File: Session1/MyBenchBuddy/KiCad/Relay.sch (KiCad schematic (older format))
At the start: 0 parts

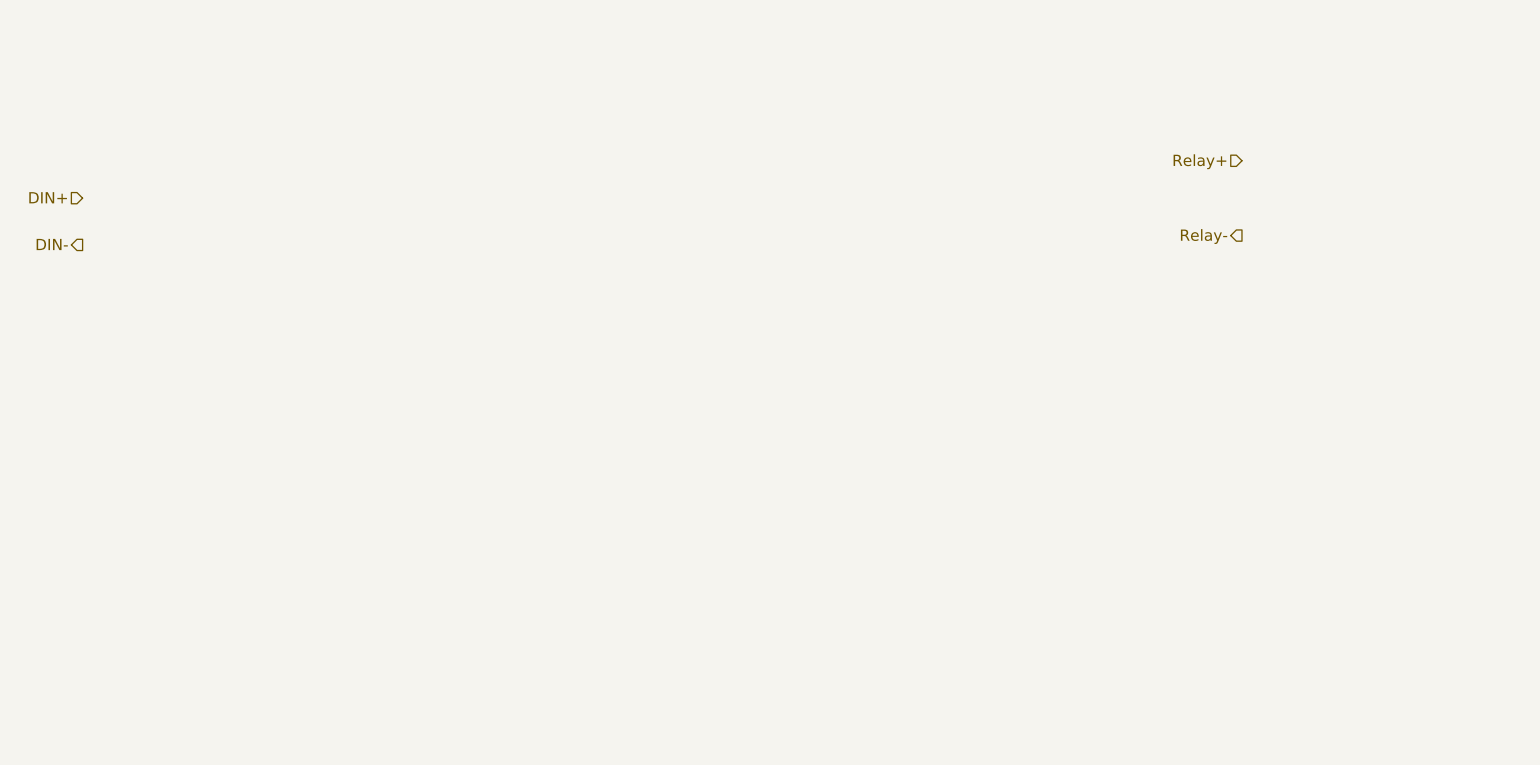
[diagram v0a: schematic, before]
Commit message: Module3Unit5
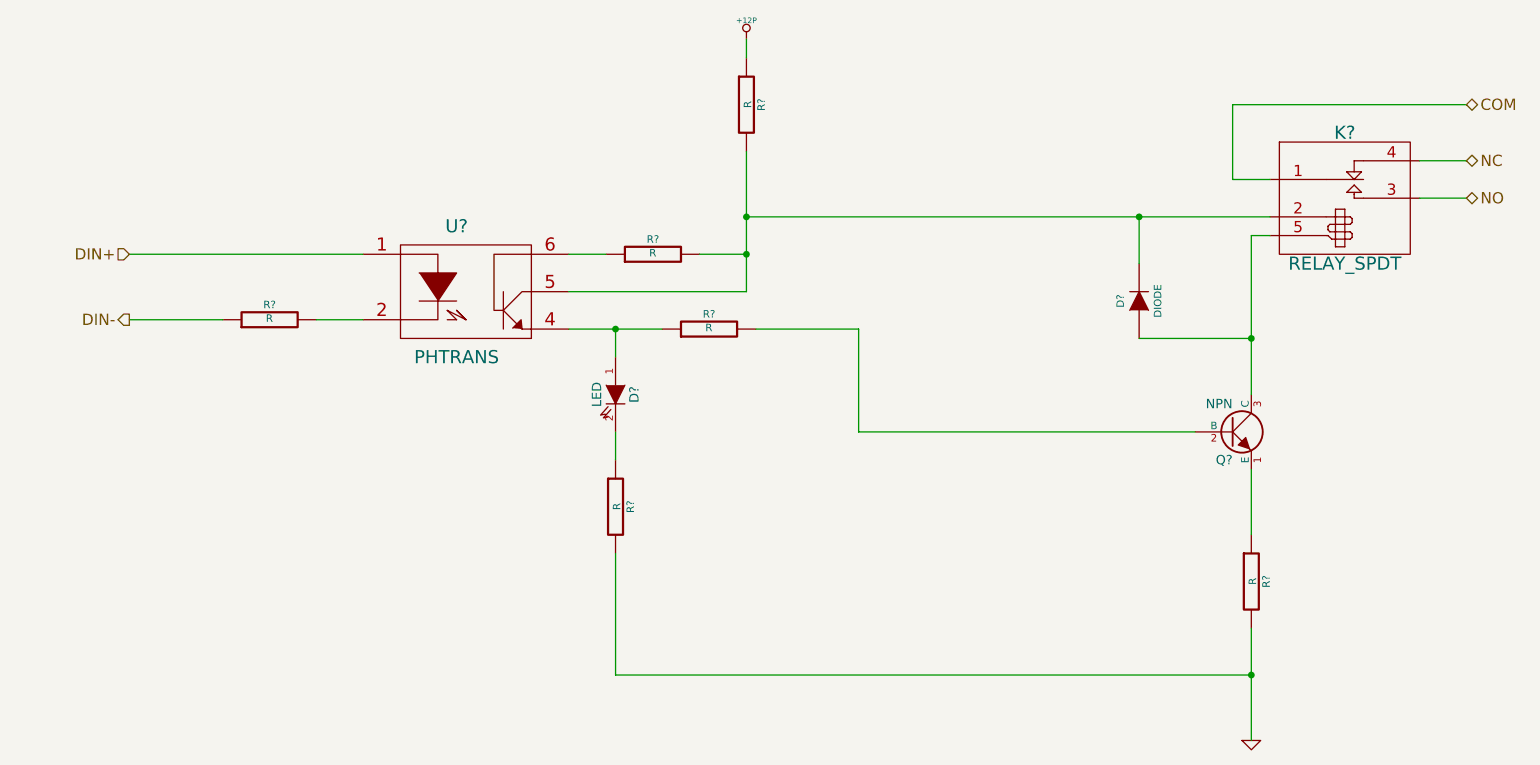
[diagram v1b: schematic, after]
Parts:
- added D?: LED, symbol LED
- added D?: DIODE, symbol DIODE
- added K?: RELAY_SPDT, symbol RELAY_SPDT
- added Q?: NPN, symbol NPN
- added R? (x6): R, symbol R
- added U?: PHTRANS, symbol PHTRANS
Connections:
- net DIN+: now also U?.1
- net DIN-: now also R?.1
- new net: R?.2, U?.2
- new net: D?.1 (A), R?.1, U?.4
- new net: D?.2 (K), K?.2 (COIL+), R?.2, R?.2, U?.5
- new net: R?.1, U?.6
- new net: Q?.2 (B), R?.2
- new net: Q?.1 (E), R?.1
- new net: D?.1 (A), K?.5 (COIL-), Q?.3 (C)
- new net: D?.2 (K), R?.1
- new net +12P: R?.1
- new net COM: K?.1 (COM)
- new net GND: R?.2, R?.2
- new net NC: K?.4 (NC)
- new net NO: K?.3 (NO)
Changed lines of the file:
@@
 LIBS:contrib
 LIBS:valves
+LIBS:bth-switch
 LIBS:MyBenchBuddy-cache
 EELAYER 24 0
@@
 $Descr A4 11693 8268
 encoding utf-8
-Sheet 4 8
+Sheet 8 8
 Title ""
 Date ""
@@
 Comment4 ""
 $EndDescr
-Text HLabel 2450 2400 0    60   Input ~ 0
+Text HLabel 2700 2700 0    60   Input ~ 0
 DIN+
-Text HLabel 2450 2650 0    60   Output ~ 0
+Text HLabel 2700 3050 0    60   Output ~ 0
 DIN-
-Text HLabel 8650 2200 0    60   Input ~ 0
-Relay+
-Text HLabel 8650 2600 0    60   Output ~ 0
-Relay-
+Text HLabel 9850 2200 2    60   BiDi ~ 0
+NC
+Text HLabel 9850 2400 2    60   BiDi ~ 0
+NO
+$Comp
+L PHTRANS U?
+U 1 1 52465652
+P 4500 2900
+F 0 "U?" H 4450 3250 70  0000 C CNN
+F 1 "PHTRANS" H 4450 2550 70  0000 C CNN
+F 2 "" H 4500 2900 60  0000 C CNN
+F 3 "" H 4500 2900 60  0000 C CNN
+	1    4500 2900
+	1    0    0    -1
+$EndComp
+$Comp
+L R R?
+U 1 1 52465670
+P 5800 3100
+F 0 "R?" V 5880 3100 40  0000 C CNN
+F 1 "R" V 5807 3101 40  0000 C CNN
+F 2 "" V 5730 3100 30  0000 C CNN
+F 3 "" H 5800 3100 30  0000 C CNN
+	1    5800 3100
+	0    -1   -1   0
+$EndComp
+$Comp
+L NPN Q?
+U 1 1 52465684
+P 8600 3650
+F 0 "Q?" H 8600 3500 50  0000 R CNN
+F 1 "NPN" H 8600 3800 50  0000 R CNN
+F 2 "" H 8600 3650 60  0000 C CNN
+F 3 "" H 8600 3650 60  0000 C CNN
+	1    8600 3650
+	1    0    0    -1
+$EndComp
+$Comp
+L LED D?
+U 1 1 52465698
+P 5300 3450
+F 0 "D?" H 5300 3550 50  0000 C CNN
+F 1 "LED" H 5300 3350 50  0000 C CNN
+F 2 "" H 5300 3450 60  0000 C CNN
+F 3 "" H 5300 3450 60  0000 C CNN
+	1    5300 3450
+	0    1    1    0
+$EndComp
+$Comp
+L RELAY_SPDT K?
+U 1 1 52465D2B
+P 9200 2250
+F 0 "K?" H 9200 2450 70  0000 C CNN
+F 1 "RELAY_SPDT" H 9200 1750 70  0000 C CNN
+F 2 "" H 9200 2250 60  0000 C CNN
+F 3 "" H 9200 2250 60  0000 C CNN
+	1    9200 2250
+	1    0    0    -1
+$EndComp
+Text HLabel 9850 1900 2    60   BiDi ~ 0
+COM
+Wire Wire Line
+	9850 2200 9600 2200
+Wire Wire Line
+	9850 2400 9600 2400
+Wire Wire Line
+	5050 3100 5550 3100
+Wire Wire Line
+	8700 3850 8700 4200
+Wire Wire Line
+	8800 2500 6000 2500
+Wire Wire Line
+	6000 2150 6000 2900
+$Comp
+L R R?
+U 1 1 52466639
+P 8700 4450
+F 0 "R?" V 8780 4450 40  0000 C CNN
+F 1 "R" V 8707 4451 40  0000 C CNN
+F 2 "" V 8630 4450 30  0000 C CNN
+F 3 "" H 8700 4450 30  0000 C CNN
+	1    8700 4450
+	1    0    0    -1
+$EndComp
+$Comp
+L GND #PWR?
+U 1 1 52466775
+P 8700 5300
+F 0 "#PWR?" H 8700 5300 30  0001 C CNN
+F 1 "GND" H 8700 5230 30  0001 C CNN
+F 2 "" H 8700 5300 60  0000 C CNN
+F 3 "" H 8700 5300 60  0000 C CNN
+	1    8700 5300
+	1    0    0    -1
+$EndComp
+Wire Wire Line
+	8700 4700 8700 5300
+$Comp
+L R R?
+U 1 1 524668CF
+P 5300 4050
+F 0 "R?" V 5380 4050 40  0000 C CNN
+F 1 "R" V 5307 4051 40  0000 C CNN
+F 2 "" V 5230 4050 30  0000 C CNN
+F 3 "" H 5300 4050 30  0000 C CNN
+	1    5300 4050
+	1    0    0    -1
+$EndComp
+Wire Wire Line
+	5300 3100 5300 3250
+Connection ~ 5300 3100
+Wire Wire Line
+	5300 3650 5300 3800
+Connection ~ 8700 4950
+$Comp
+L R R?
+U 1 1 52466A3B
+P 6000 1900
+F 0 "R?" V 6080 1900 40  0000 C CNN
+F 1 "R" V 6007 1901 40  0000 C CNN
+F 2 "" V 5930 1900 30  0000 C CNN
+F 3 "" H 6000 1900 30  0000 C CNN
+	1    6000 1900
+	1    0    0    -1
+$EndComp
+$Comp
+L +12P #PWR?
+U 1 1 52466A48
+P 6000 1550
+F 0 "#PWR?" H 6000 1520 30  0001 C CNN
+F 1 "+12P" H 6000 1650 30  0000 C CNN
+F 2 "" H 6000 1550 60  0000 C CNN
+F 3 "" H 6000 1550 60  0000 C CNN
+	1    6000 1550
+	1    0    0    -1
+$EndComp
+Wire Wire Line
+	6000 1650 6000 1550
+Wire Wire Line
+	6000 2900 5050 2900
+Connection ~ 6000 2500
+$Comp
+L R R?
+U 1 1 52466CFF
+P 5500 2700
+F 0 "R?" V 5580 2700 40  0000 C CNN
+F 1 "R" V 5507 2701 40  0000 C CNN
+F 2 "" V 5430 2700 30  0000 C CNN
+F 3 "" H 5500 2700 30  0000 C CNN
+	1    5500 2700
+	0    -1   -1   0
+$EndComp
+Wire Wire Line
+	5050 2700 5250 2700
+Wire Wire Line
+	5750 2700 6000 2700
+Connection ~ 6000 2700
+$Comp
+L R R?
+U 1 1 52466E75
+P 3450 3050
+F 0 "R?" V 3530 3050 40  0000 C CNN
+F 1 "R" V 3457 3051 40  0000 C CNN
+F 2 "" V 3380 3050 30  0000 C CNN
+F 3 "" H 3450 3050 30  0000 C CNN
+	1    3450 3050
+	0    -1   -1   0
+$EndComp
+Wire Wire Line
+	3700 3050 3950 3050
+Wire Wire Line
+	2700 3050 3200 3050
+Wire Wire Line
+	2700 2700 3950 2700
+Wire Wire Line
+	9850 1900 8600 1900
+Wire Wire Line
+	8600 1900 8600 2300
+Wire Wire Line
+	8600 2300 8800 2300
+Wire Wire Line
+	8800 2600 8700 2600
+Wire Wire Line
+	8700 2600 8700 3450
+$Comp
+L DIODE D?
+U 1 1 52467327
+P 8100 2950
+F 0 "D?" H 8100 3050 40  0000 C CNN
+F 1 "DIODE" H 8100 2850 40  0000 C CNN
+F 2 "" H 8100 2950 60  0000 C CNN
+F 3 "" H 8100 2950 60  0000 C CNN
+	1    8100 2950
+	0    -1   -1   0
+$EndComp
+Wire Wire Line
+	8400 3650 6600 3650
+Wire Wire Line
+	6600 3650 6600 3100
+Wire Wire Line
+	6600 3100 6050 3100
+Wire Wire Line
+	8700 4950 5300 4950
+Wire Wire Line
+	5300 4950 5300 4300
+Wire Wire Line
+	8100 2500 8100 2750
+Connection ~ 8100 2500
+Wire Wire Line
+	8100 3150 8700 3150
+Connection ~ 8700 3150
 $EndSCHEMATC
